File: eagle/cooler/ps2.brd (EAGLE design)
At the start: 228.6 x 152.4 mm, 18 parts, among them IC5 7812TV, J1 PIN2F061.100, J2 PIN2F061.100, J3 PIN2F061.100, J4 PIN2F061.100, J5 PIN2F061.100, J6 PIN2F061.100, Q1 2N5883, T1 2N3055, T2 2N3055

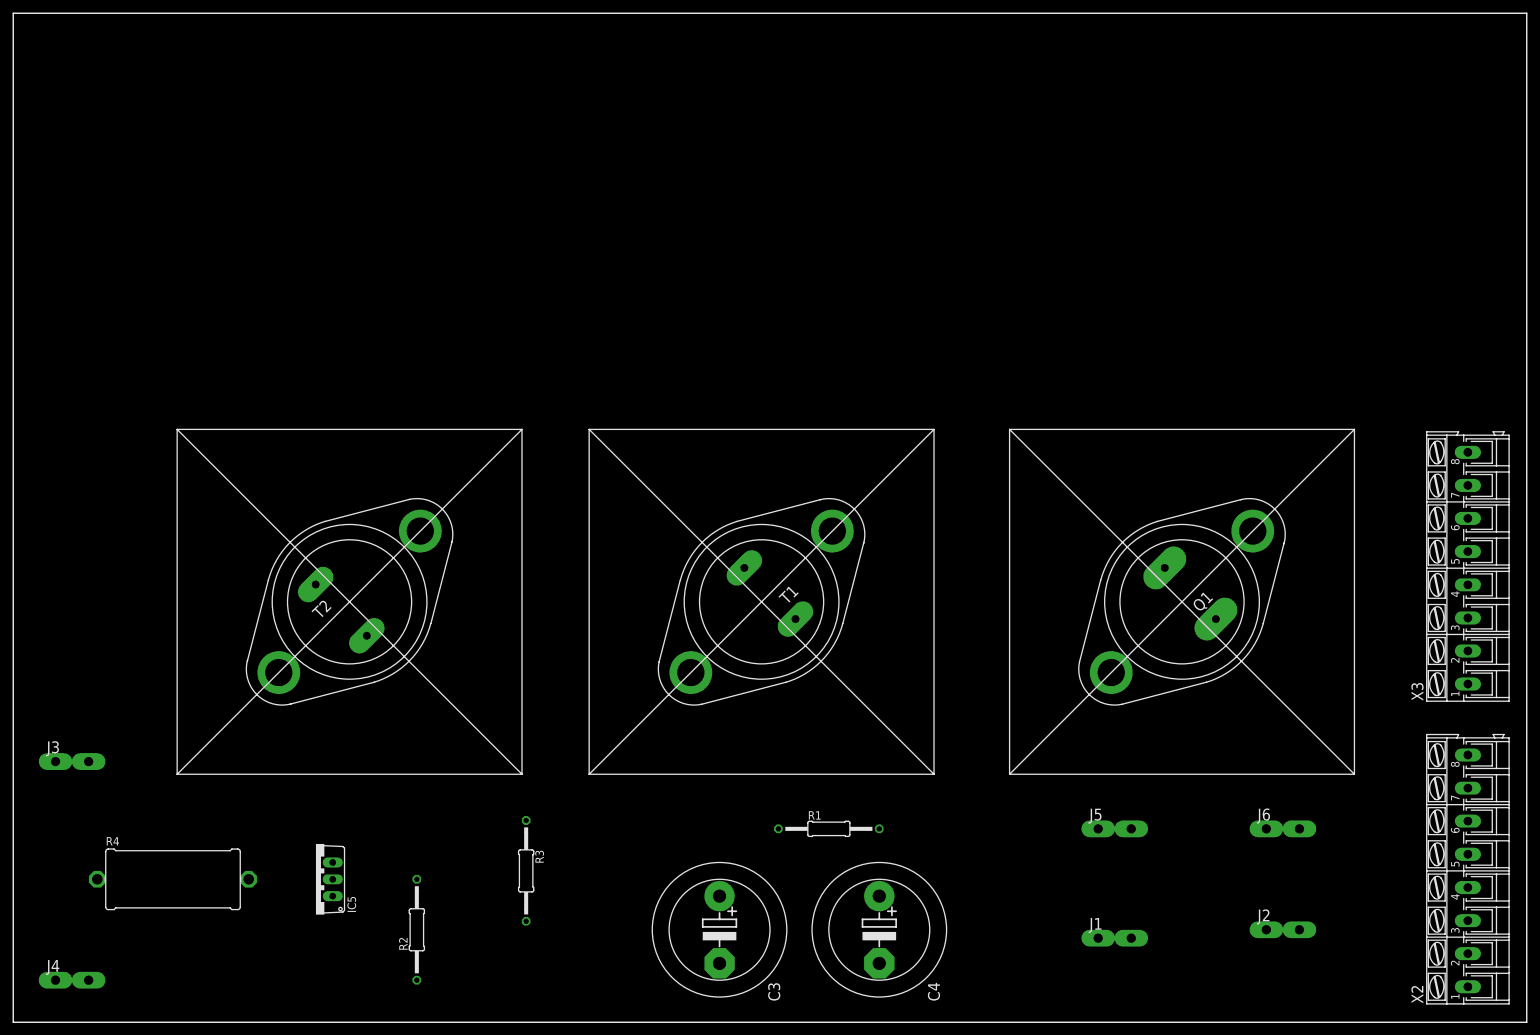
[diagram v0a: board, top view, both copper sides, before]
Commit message: layouts
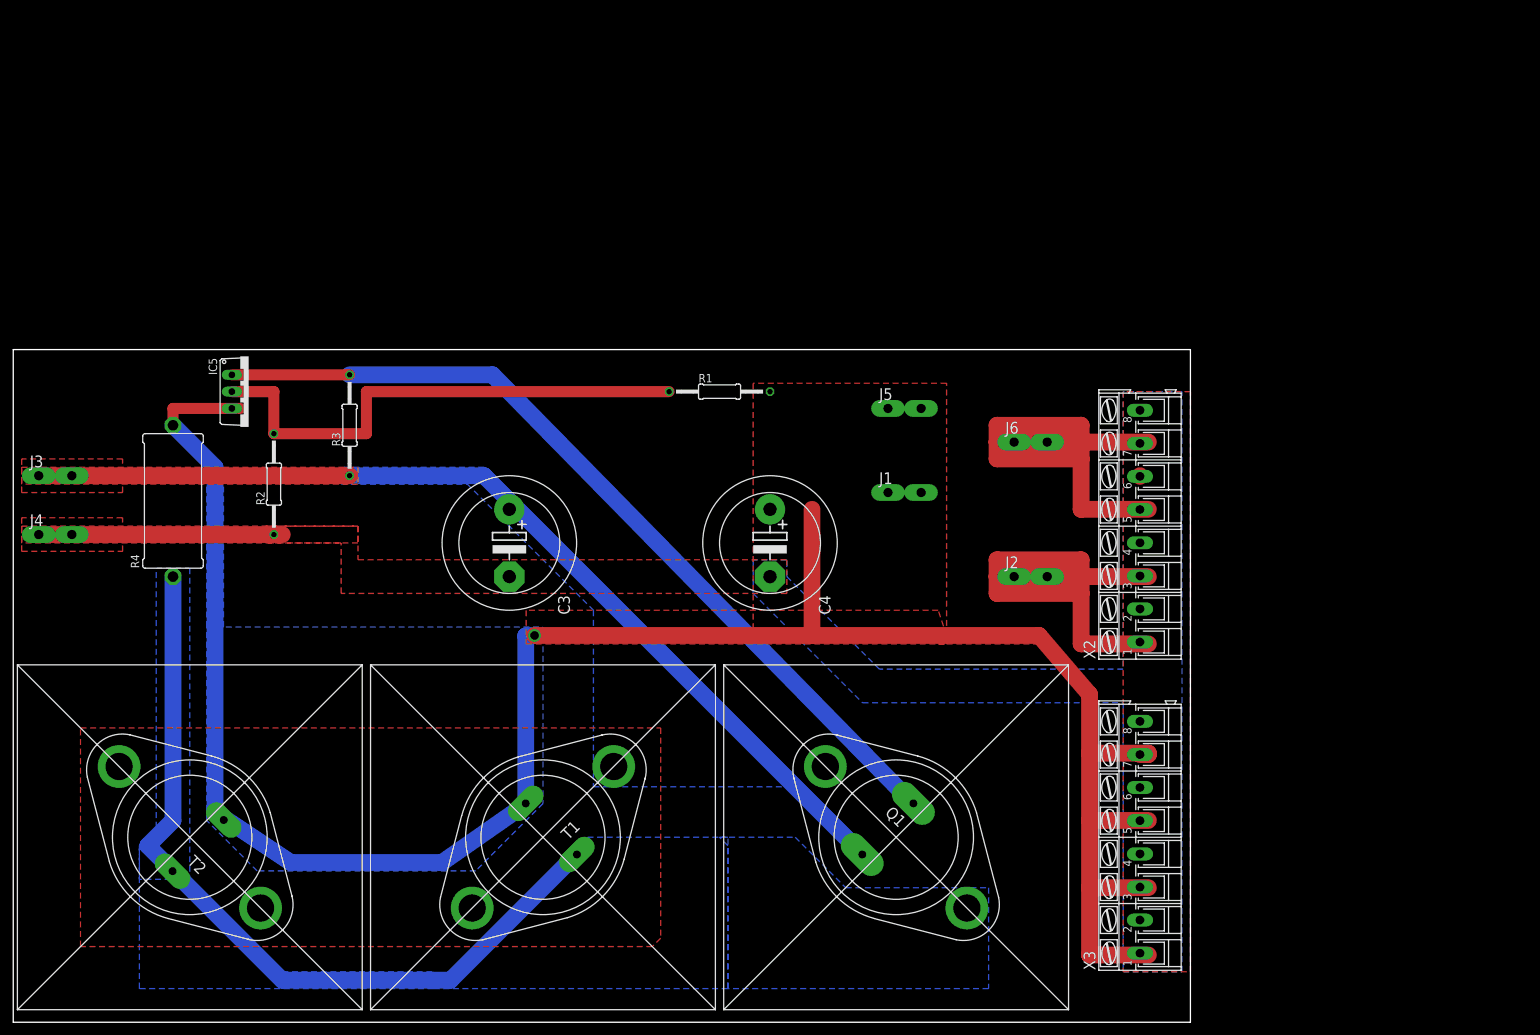
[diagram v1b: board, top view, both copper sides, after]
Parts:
- moved J1 74.4 mm to (134.6, 80.0)
- moved IC5 74.4 mm to (35.6, 95.2), turned to 270 degrees
- moved R3 72.4 mm to (50.8, 90.2), turned to 90 degrees
- moved X2 71.9 mm to (170.2, 74.9)
- moved J5 71.0 mm to (134.6, 92.7)
- moved R2 70.7 mm to (39.4, 81.3)
- moved J6 69.7 mm to (153.7, 87.6)
- moved R1 68.1 mm to (106.7, 95.2)
- moved J4 67.4 mm to (6.35, 73.7)
- moved C3 66.5 mm to (74.9, 72.4)
- moved J2 65.5 mm to (153.7, 67.3)
- moved X3 64.1 mm to (170.2, 27.9)
- moved C4 60.7 mm to (114.3, 72.4)
- moved R4 57.1 mm to (24.1, 78.7), turned to 90 degrees
- moved Q1 55.9 mm to (133.3, 27.9), turned to 315 degrees
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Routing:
- net VDD: track 0.00 -> 335.9 mm, vias 0 -> 1
- net VIN: track 0.00 -> 149.9 mm
- net N$4: track 0.00 -> 131.9 mm
- net N$1: track 0.00 -> 125.1 mm
- net N$5: track 0.00 -> 78.7 mm
- net TEC1: track 0.00 -> 76.2 mm
- net TEC2: track 0.00 -> 74.9 mm
- net GND: track 0.00 -> 36.9 mm
- added copper zone on layer 1, net GND
- added copper zone on layer 16, net GND
- added copper zone on layer 16, net N$1
- added copper zone on layer 1, net VDD
- added copper zone on layer 16, net VDD
- added copper zone on layer 1, net VIN
- added copper zone on layer 16, net VIN
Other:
- board size 228.6 x 152.4 mm -> 177.8 x 101.6 mm
